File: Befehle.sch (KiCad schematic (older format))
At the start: 66 parts

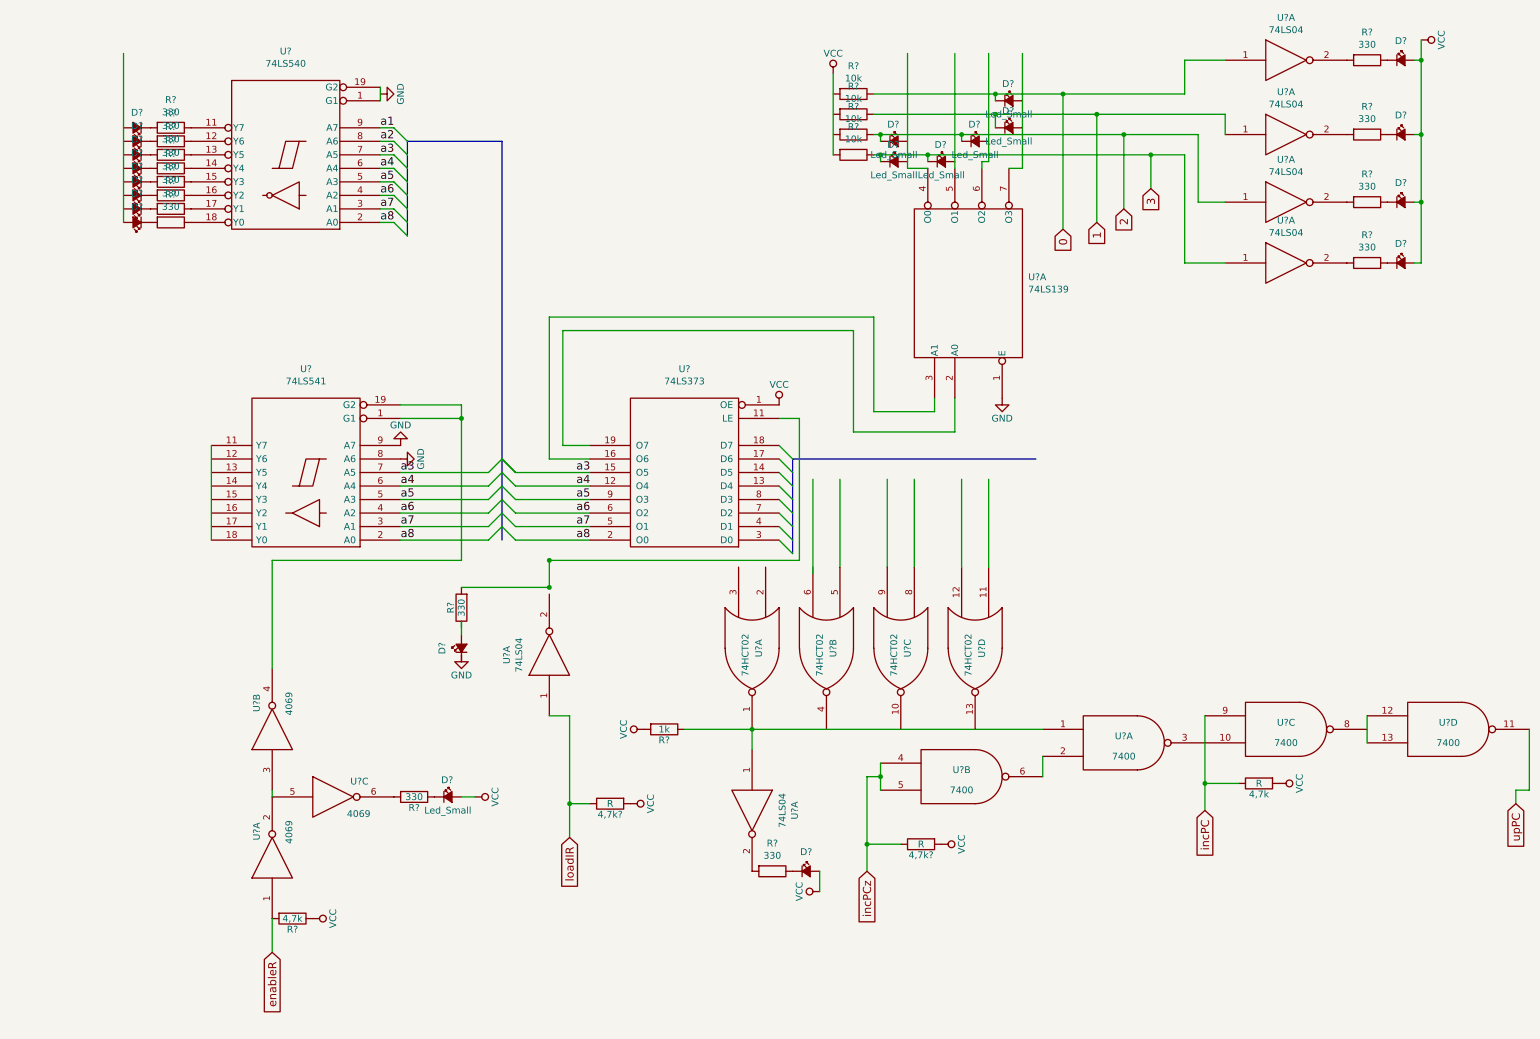
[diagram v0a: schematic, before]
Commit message: Befehle Speicherplan fast fertig
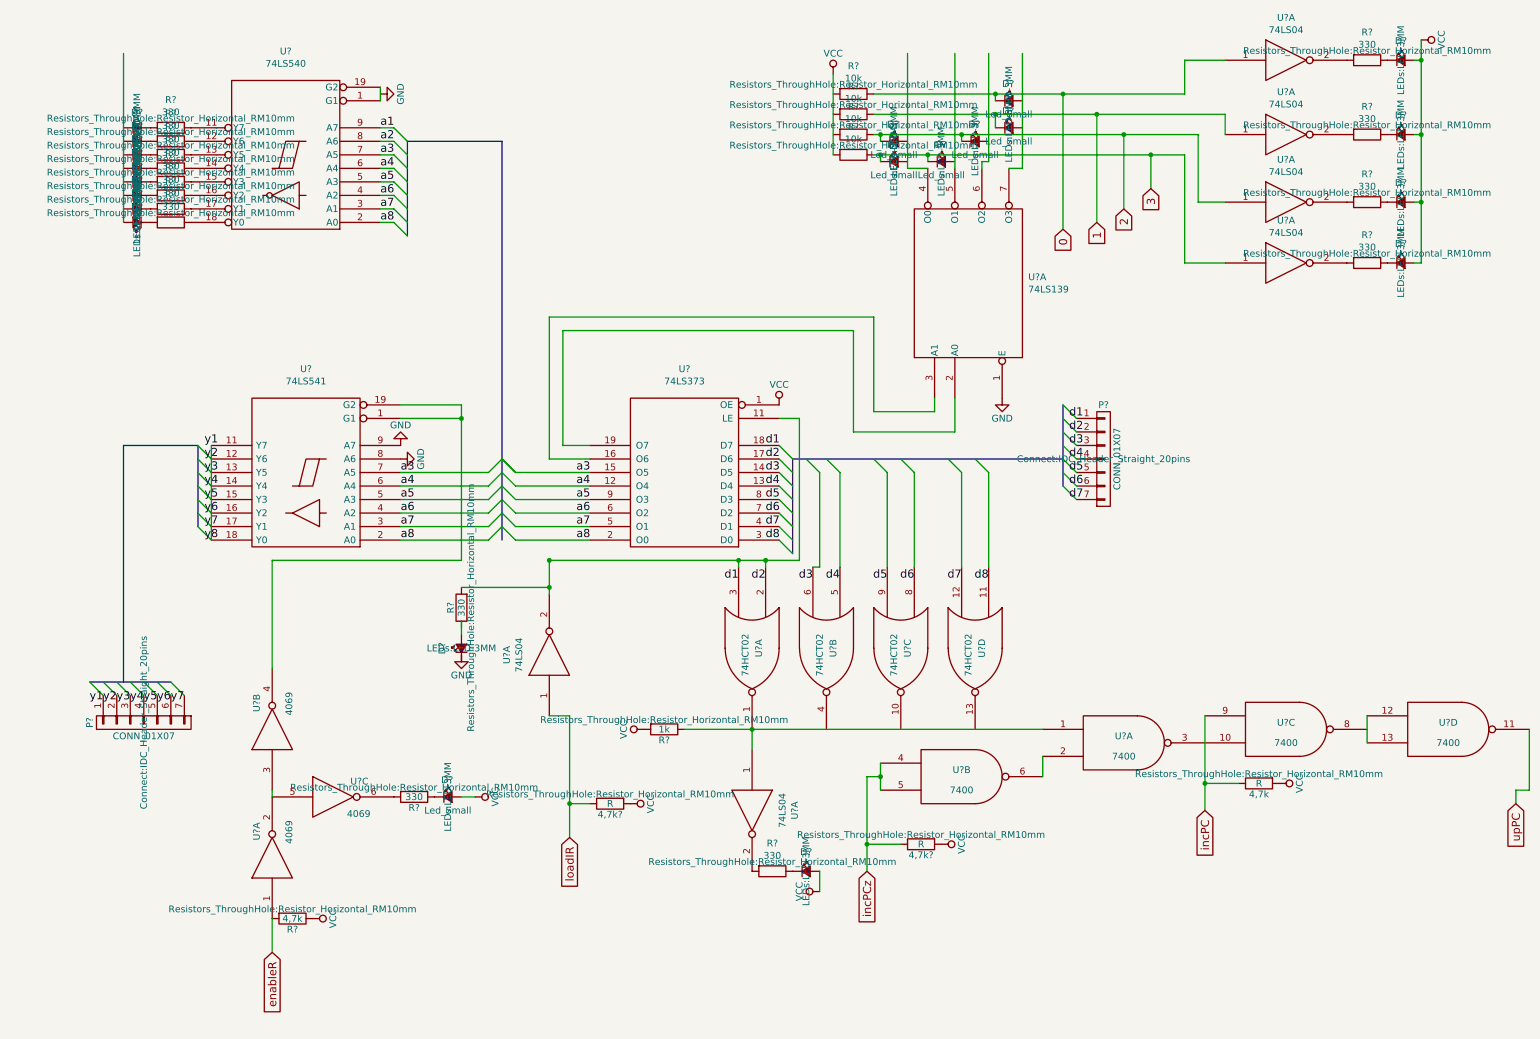
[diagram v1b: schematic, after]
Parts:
- added P? (x2): CONN_01X07, Connect:IDC_Header_Straight_20pins, symbol CONN_01X07
- 4,7k, 4,7k? (x2), R? (x21): footprint (none) -> Resistors_ThroughHole:Resistor_Horizontal_RM10mm
- D? (x21): footprint (none) -> LEDs:LED-3MM
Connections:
- net labels added: d1, d2, d3, d4, d5, d6, d7, d8, y1, y2, y3, y4, y5, y6, y7, y8
- wire segments 107 -> 110
